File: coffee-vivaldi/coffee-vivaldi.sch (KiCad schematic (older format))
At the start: 69 parts, among them J1 Conn_Coaxial, J2 AudioPlug3, SW1 SW_SPDT, U1 Opamp_Quad_Generic, U3 OPA1604

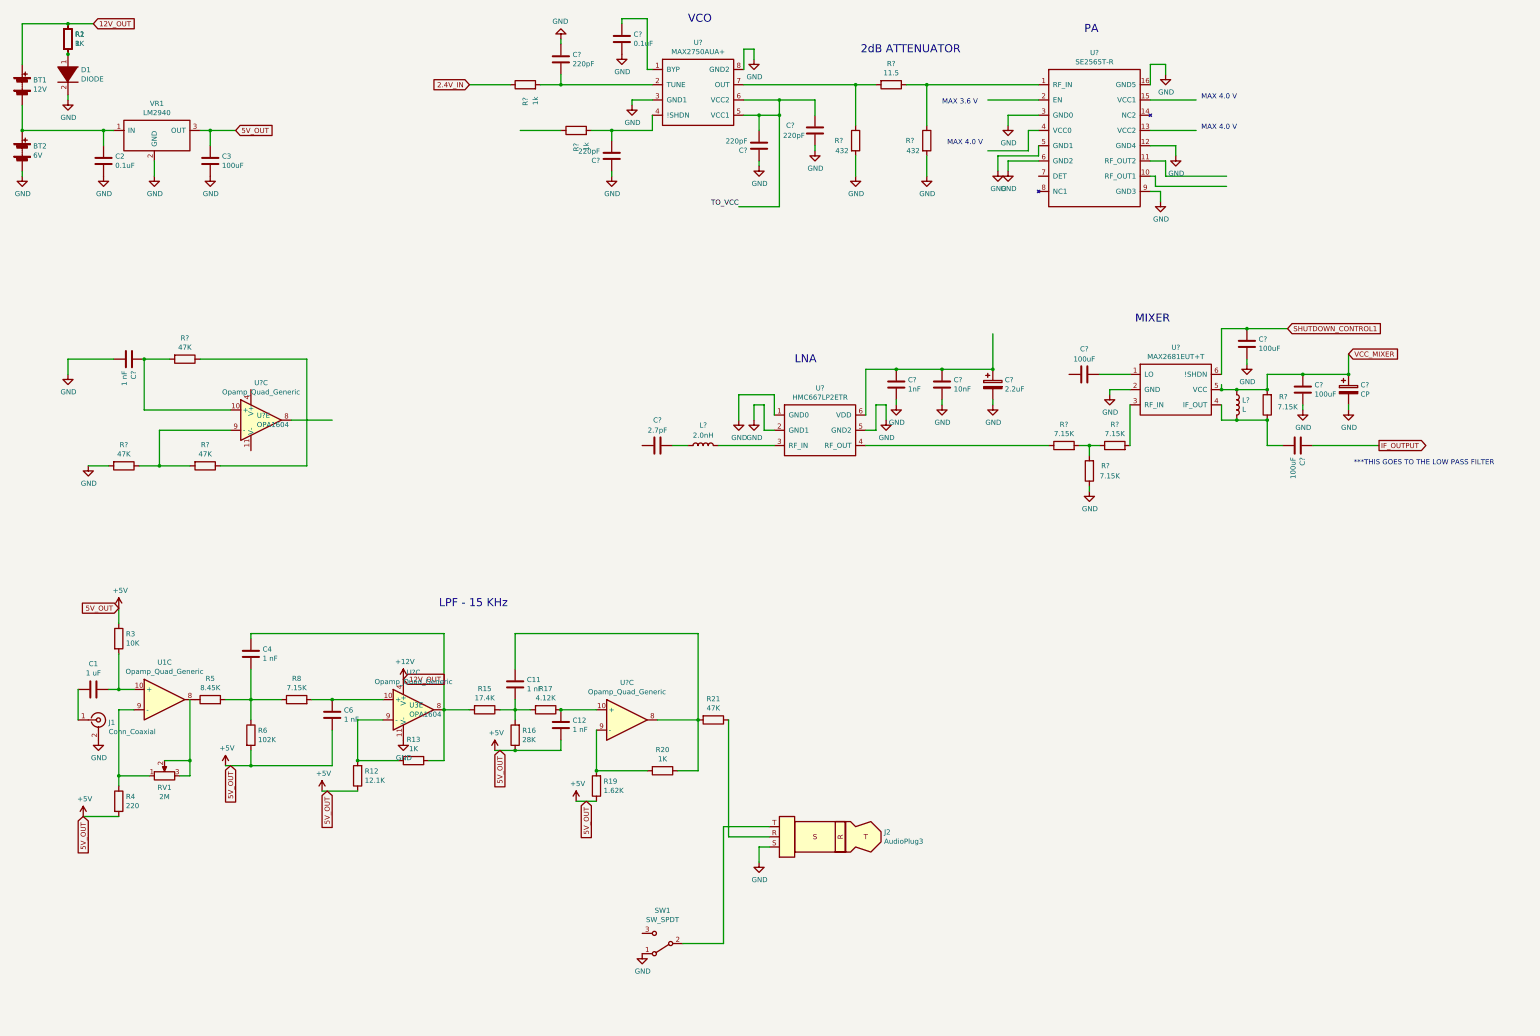
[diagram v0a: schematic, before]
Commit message: Edited radar schematic
Still a work in progress.
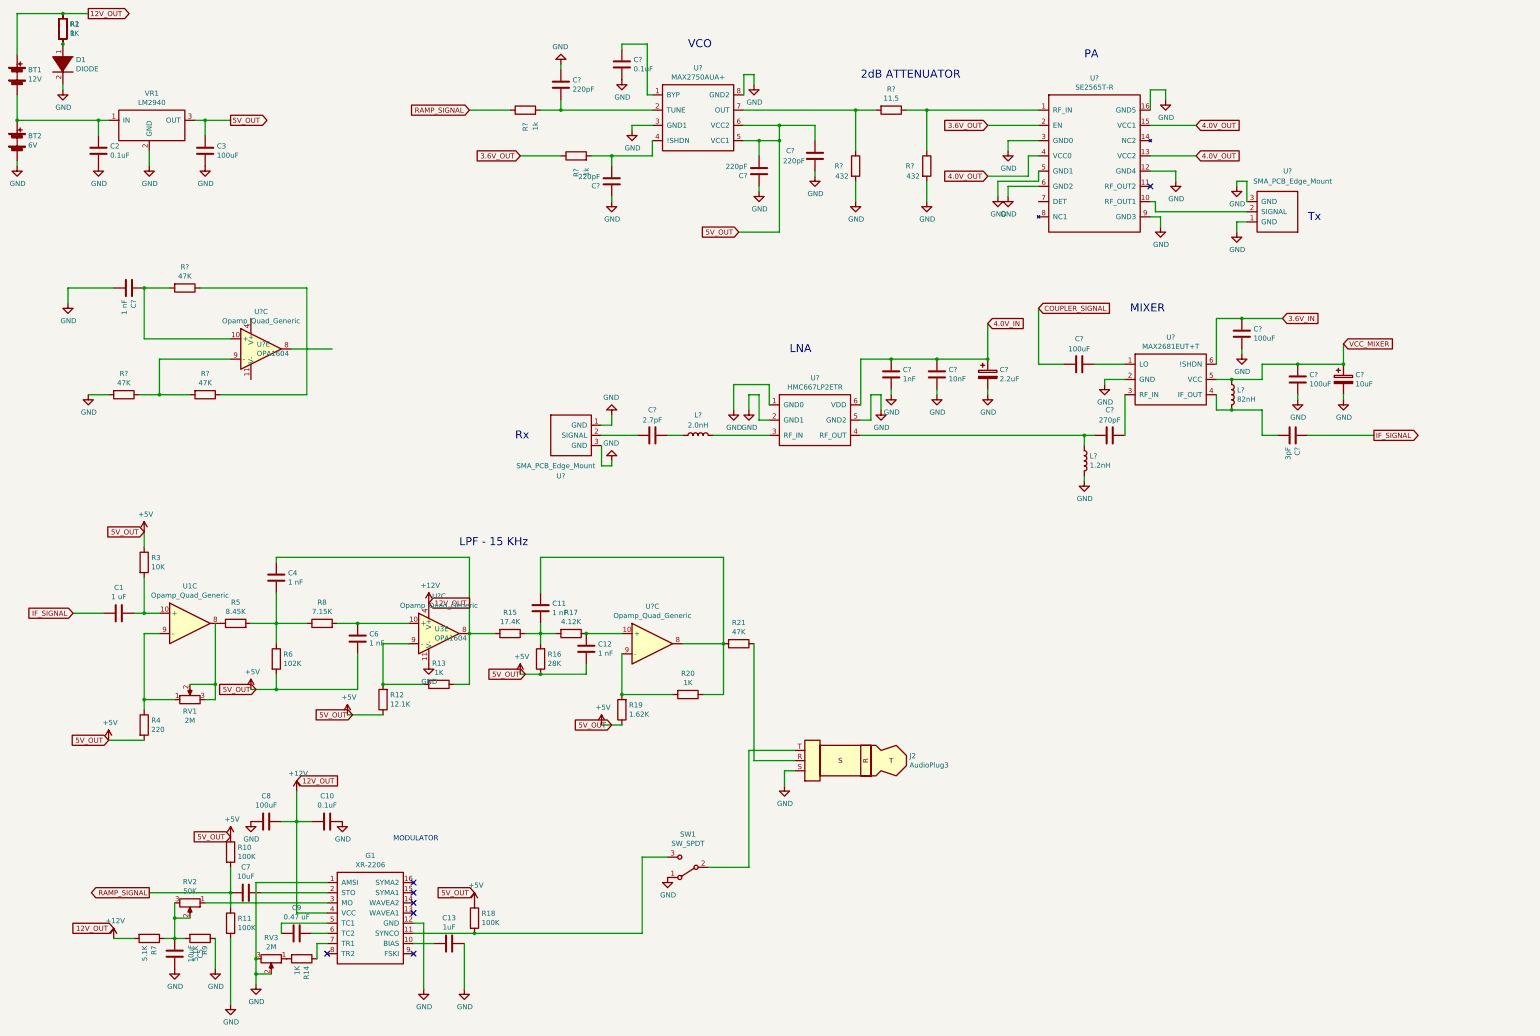
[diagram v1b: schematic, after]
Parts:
- removed J1: Conn_Coaxial, symbol Connector:Conn_Coaxial
- removed R? (x4): 7.15K, symbol Device:R
- removed U?: HMC667LP2ETR, symbol coffee-vivaldi-rescue:HMC667LP2ETR-coffee-vivaldi-cache
- removed U?: Opamp_Quad_Generic, symbol Device:Opamp_Quad_Generic
- removed U?: MAX2681EUT+T, symbol coffee-vivaldi-rescue:MAX2681EUT+T-coffee-vivaldi-cache
- removed U?: MAX2750AUA+, symbol coffee-vivaldi-rescue:MAX2750AUA+-coffee-vivaldi-cache
- removed U?: SE2565T-R, symbol coffee-vivaldi-rescue:SE2565T-R-coffee-vivaldi-cache
- added C10: 0.1uF, symbol Device:C
- added C13: 1uF, symbol Device:C
- added C5, C7: 10uF, symbol Device:C
- added C8: 100uF, symbol Device:C
- added C9: 0.47 uF, symbol Device:C
- added C?: 270pF, symbol Device:C
- added G1: XR-2206, symbol HS2_Parts:XR-2206
- added L?: 1.2nH, symbol Device:L
- added R10, R11, R18: 100K, symbol Device:R
- added R14: 1K, symbol Device:R
- added R7, R9: 5.1K, symbol Device:R
- added RV2: 50K, symbol Device:R_POT
- added RV3: 2M, symbol Device:R_POT
- added U?: MAX2681EUT+T, symbol HS2_Parts:MAX2681EUT+T
- added U?: HMC667LP2ETR, symbol HS2_Parts:HMC667LP2ETR
- added U?: MAX2750AUA+, symbol HS2_Parts:MAX2750AUA+
- added U?: SE2565T-R, symbol HS2_Parts:SE2565T-R
- added U? (x2): SMA_PCB_Edge_Mount, symbol HS2_Parts:SMA_PCB_Edge_Mount
- added U?: Opamp_Quad_Generic, symbol Device:Opamp_Quad_Generic
- C?: value 100uF -> 3pF
- C?: value CP -> 10uF
- L?: value L -> 82nH
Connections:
- net labels added: 3.6V_IN, 3.6V_OUT, 4.0V_IN, 4.0V_OUT, COUPLER_SIGNAL, IF_SIGNAL, RAMP_SIGNAL
- net labels removed: 2.4V_IN, IF_OUTPUT, SHUTDOWN_CONTROL1, TO_VCC
- wire segments 199 -> 243
- no-connect marks 0 -> 7
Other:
- note added: "MODULATOR"
- note added: "Rx"
- note added: "Tx"
- note removed: "***THIS GOES TO THE LOW PASS FILTER"
- note removed: "MAX 3.6 V"
- note removed: "MAX 4.0 V"
- moved on the sheet: C1, C6, C?, L?, R21, R3, R4, R6, R8, R?, SW1, U1C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
